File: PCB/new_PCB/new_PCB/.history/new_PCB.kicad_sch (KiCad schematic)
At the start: 54 parts, among them J1 XT60PW-F, J2 XT60PW-F, J3 MOLEX-Connector, J4 MOLEX-Connector, J5 MOLEX-Connector, J6 MOLEX-Connector, J7 MOLEX-Connector, J8 MOLEX-Connector, Q1 Q_PMOS, Q2 Q_PMOS, SW1 SW_SPDT, U1 ESP32-S3-DEVKITC-1-N16R8V

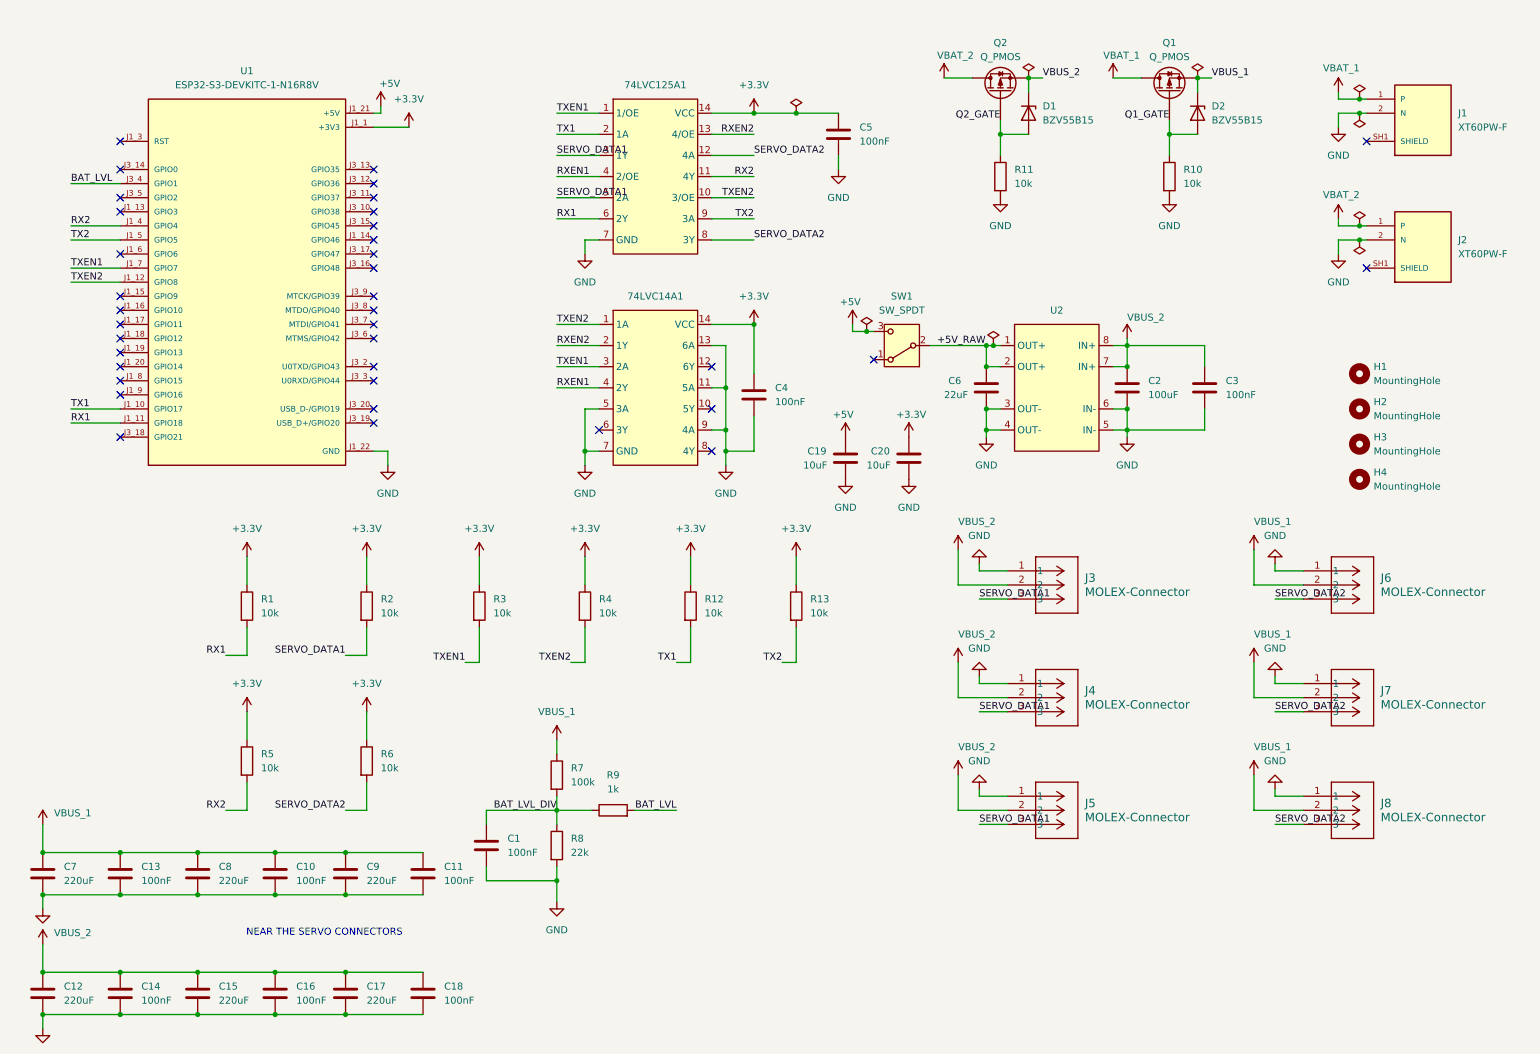
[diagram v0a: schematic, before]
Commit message: Final version of 2.0 PCB version
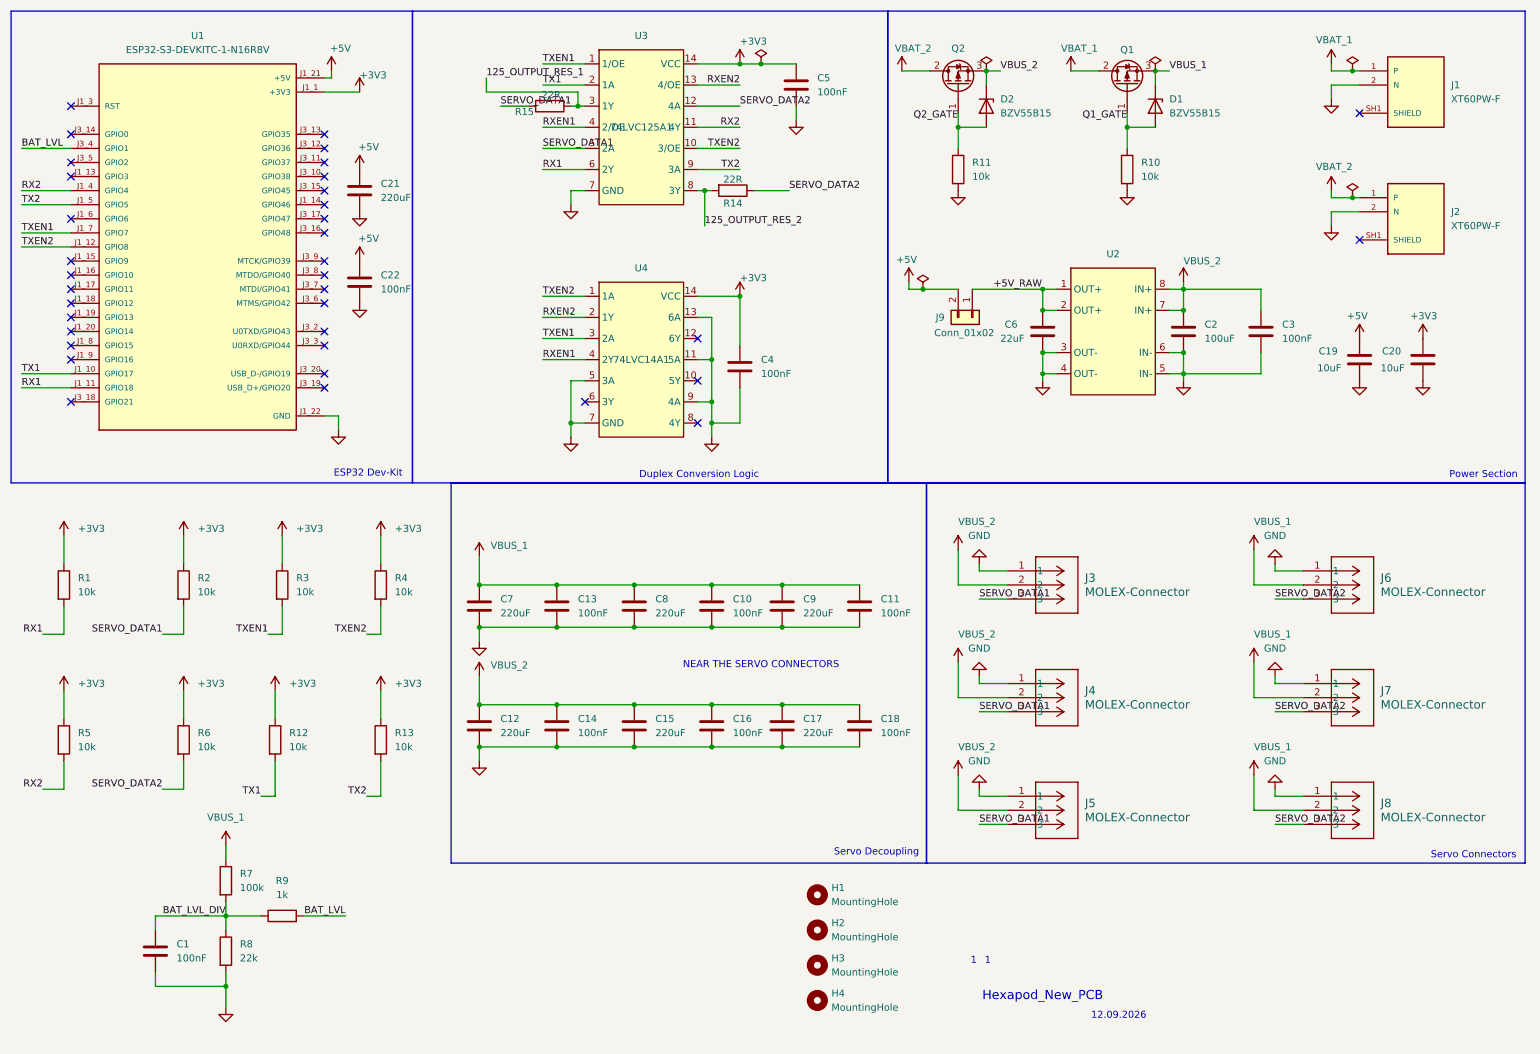
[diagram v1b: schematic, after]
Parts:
- removed Q1, Q2: Q_PMOS, Package_TO_SOT_SMD:TO-252-2, symbol Device:Q_PMOS
- removed SW1: SW_SPDT, Elements:SW_Toggle_SPDT_TST1D_2.54mm, symbol Switch:SW_SPDT
- added C21: 220uF, Capacitor_THT:CP_Radial_D6.3mm_P2.50mm, symbol Device:C
- added C22: 100nF, Capacitor_SMD:C_0805_2012Metric, symbol Device:C
- added J9: Conn_01x02, Connector_PinHeader_2.54mm:PinHeader_1x02_P2.54mm_Vertical, symbol Connector_Generic:Conn_01x02
- added Q1, Q2: SUD50P04-08, Package_TO_SOT_SMD:TO-252-2, symbol Transistor_FET:SUD50P04-08
- added R14, R15: 22R, Resistor_SMD:R_0805_2012Metric_Pad1.20x1.40mm_HandSolder, symbol Device:R
- C19, C20: footprint Capacitor_THT:CP_Radial_D6.3mm_P2.50mm -> Capacitor_SMD:C_0805_2012Metric
- J1, J2: footprint Elements:AMASS_XT60PW-F -> Elements:AMASS-XT60PW-F
- U3: renamed from 74LVC125A1; value (none) -> 74LVC125A1
- U4: renamed from 74LVC14A1; value (none) -> 74LVC14A1
- renumbered D2 to D1, D1 to D2
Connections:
- net +5V: now also C21.1, C22.1, J9.2 (Pin_2)
- net +5V_RAW: now also J9.1 (Pin_1)
- net GND: now also C21.2, C22.2
- net Q1_GATE: now also Q1.1 (G)
- net Q2_GATE: now also Q2.1 (G)
- net SERVO_DATA1: now also R15.2; no longer U3.3 (1Y)
- net SERVO_DATA2: now also R14.1; no longer U3.8 (3Y)
- net VBAT_1: now also Q1.2 (D)
- net VBAT_2: now also Q2.2 (D)
- net VBUS_1: now also Q1.3 (S)
- net VBUS_2: now also Q2.3 (S)
- net +3.3V renamed +3V3
- new net 125_OUTPUT_RES_1: R15.1, U3.3 (1Y)
- new net 125_OUTPUT_RES_2: R14.2, U3.8 (3Y)
- no-connect marks 37 -> 36
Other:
- note added: "1"
- note added: "12.09.2026"
- note added: "Duplex Conversion Logic"
- note added: "ESP32 Dev-Kit"
- note added: "Hexapod_New_PCB"
- note added: "Power Section"
- note added: "Servo Connectors"
- note added: "Servo Decoupling"
- moved on the sheet: C1, C10, C11, C12, C13, C14, C15, C16, C17, C18, C2, C3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
